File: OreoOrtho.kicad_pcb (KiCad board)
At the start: 2 copper layers, 57.1 x 39.3 mm, 36 parts, among them SW1 MXSwitch, SW2 MXSwitch, SW3 MXSwitch, SW4 MXSwitch, SW5 MXSwitch, SW6 MXSwitch, U1 ATmega32U2-AU, U2 PRTR5V0U2X, Y1 16MHz

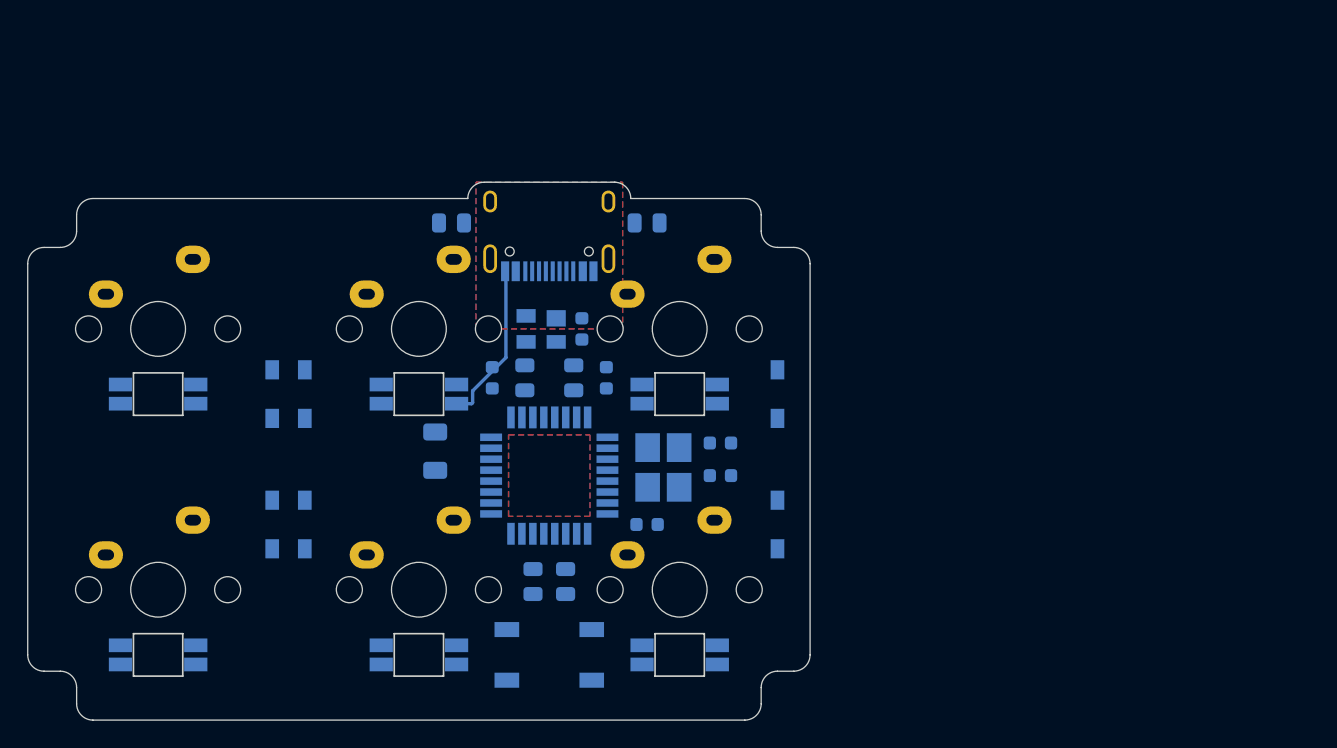
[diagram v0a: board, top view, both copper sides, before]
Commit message: made gerbers
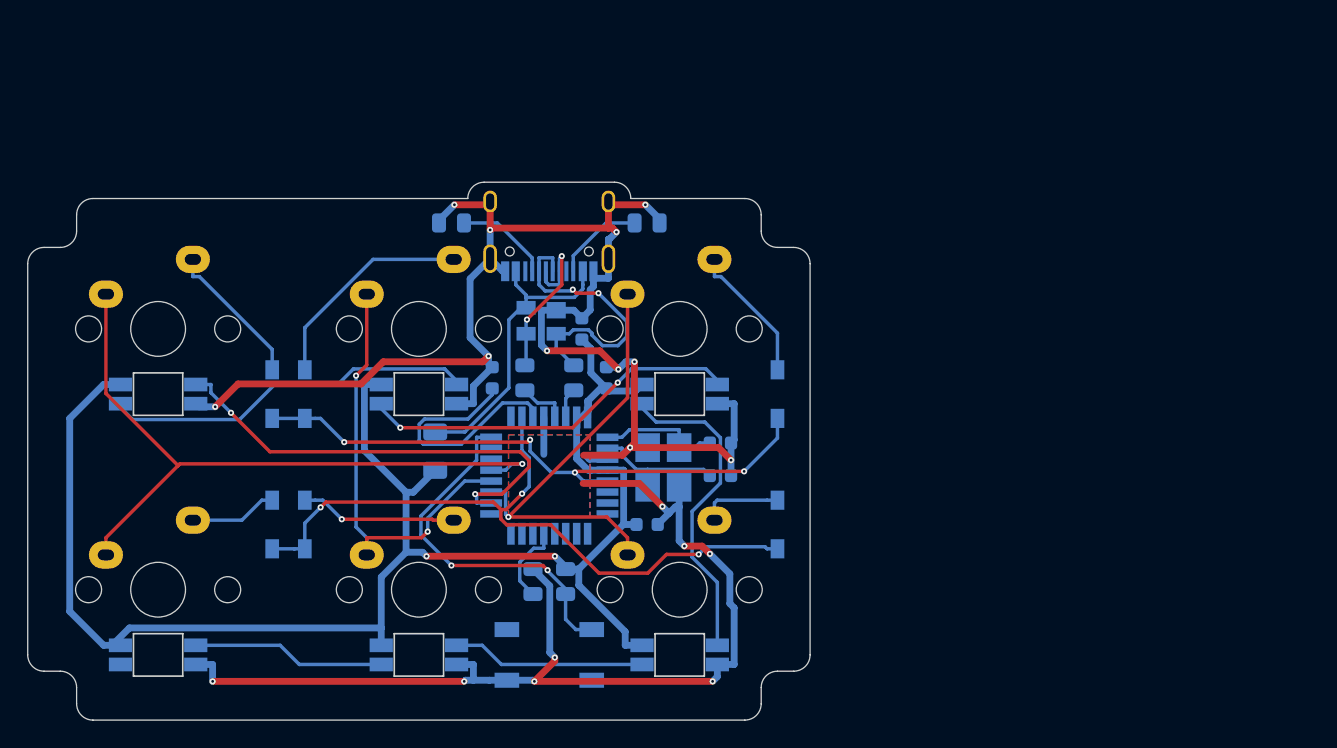
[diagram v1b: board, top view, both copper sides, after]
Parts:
- USB1: value HRO-TYPE-C-31-M-12 -> HRO-TYPE-C-31-M-12-Assembly
- moved U2 0.60 mm to (142.3, 56.6)
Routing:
- net GND: track 11.8 -> 193.8 mm, vias 0 -> 19
- net +5V: track 0.00 -> 118.4 mm, vias 0 -> 2
- net Col0: track 0.00 -> 51.1 mm, vias 0 -> 1
- net Row1: track 0.00 -> 50.9 mm, vias 0 -> 3
- net Row0: track 0.00 -> 44.3 mm, vias 0 -> 4
- net LED: track 0.00 -> 34.0 mm, vias 0 -> 2
- net Col2: track 0.00 -> 33.4 mm, vias 0 -> 1
- net Col1: track 0.00 -> 32.3 mm, vias 0 -> 2
- net Net-(LED2-Pad2): track 0.00 -> 27.9 mm, vias 0 -> 2
- net Net-(LED1-Pad2): track 0.00 -> 27.3 mm
- net Net-(R1-Pad1): track 0.00 -> 26.5 mm, vias 0 -> 2
- net Net-(LED3-Pad2): track 0.00 -> 23.7 mm
- net VCC: track 0.00 -> 22.1 mm
- net Net-(R5-Pad2): track 0.00 -> 21.6 mm, vias 0 -> 2
- net Net-(C3-Pad2): track 0.00 -> 18.3 mm
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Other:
- net class Default: clearance 0.2 -> 0.13; trace_width 0.25 -> 0.254; via_dia 0.8 -> 0.45; via_drill 0.4 -> 0.2
- net class thick added: clearance 0.13, trace_width 0.5, via_dia 0.45, via_drill 0.2
- rule trace_clearance: 0.2 -> 0.13
- rule trace_min: 0.2 -> 0.13
- rule via_min_drill: 0.3 -> 0.2
- rule via_min_size: 0.4 -> 0.45

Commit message: route ver1
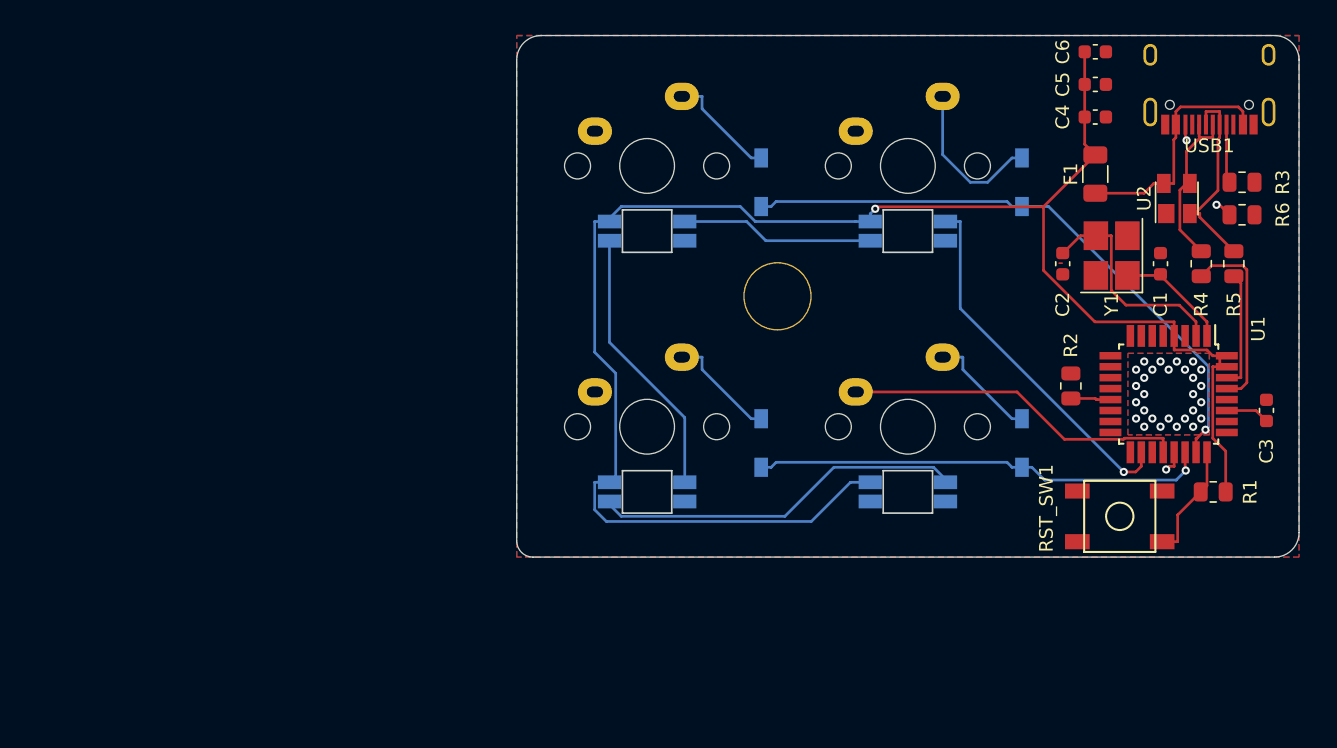
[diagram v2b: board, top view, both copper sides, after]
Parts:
- removed D5, D6: D, kbd:D3_SMD_v2
- removed LED5, LED6: YS-SK6812MINI-E, kbd:YS-SK6812MINI-E
- removed SW5, SW6: MXSwitch, kbd:CherryMX_1u
- added H1: MountingHole, kbd:HOLE, F.Cu at (159.5, 54.8)
- C1, C2, C3, C4, C5, C6, F1, R1, R2, R3, R4, R5, R6, RST_SW1, U1, U2, Y1: moved to F.Cu
- USB1: value HRO-TYPE-C-31-M-12-Assembly -> HRO-TYPE-C-31-M-12; moved to F.Cu
- moved R3 57.8 mm to (193.5, 46.4), turned to 0 degrees
- moved C3 56.6 mm to (195.3, 63.1)
- moved LED1 56.0 mm to (169.1, 50.0)
- moved SW4 56.0 mm to (169.1, 64.3)
- moved D4 55.1 mm to (177.4, 65.5)
- moved D2 54.6 mm to (177.4, 46.4)
- moved F1 52.3 mm to (182.8, 45.8), turned to 270 degrees
- moved R4 50.1 mm to (190.5, 52.4)
- moved USB1 49.4 mm to (191.1, 34.5), turned to 180 degrees
- moved R5 48.9 mm to (192.9, 52.4)
- moved R1 47.8 mm to (191.4, 69.1), turned to 0 degrees
- moved C6 47.6 mm to (182.8, 36.9)
- moved U2 47.3 mm to (188.7, 47.6), turned to 90 degrees
- moved U1 45.6 mm to (188.1, 61.9), turned to 270 degrees
- moved R6 43.5 mm to (193.5, 48.8)
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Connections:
- D3 pad 1: Row0 -> Row1
- LED4 pad 2: Net-(LED4-Pad2) -> (no net)
- SW3 pad 1: Col2 -> Col0
- SW4 pad 1: Col0 -> Col1
- U1 pad 19: Col2 -> (no net)
- U1 pad 22: (no net) -> Row1
- U1 pad 23: (no net) -> Row0
- U1 pad 26: Row1 -> (no net)
- U1 pad 5: Row0 -> (no net)
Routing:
- net GND: track 193.8 -> 0.22 mm, vias 19 -> 28
- net Col2: track 33.4 -> 0.00 mm, vias 1 -> 0
- net Net-(R1-Pad1): track 26.5 -> 8.55 mm, vias 2 -> 0
- net Row1: track 50.9 -> 33.3 mm, vias 3 -> 1
- net Net-(C3-Pad2): track 18.3 -> 3.21 mm
- net Net-(LED4-Pad2): track 14.1 -> 0.00 mm
- net Net-(LED5-Pad2): track 14.1 -> 0.00 mm
- net Col0: track 51.1 -> 64.8 mm
- net Net-(LED1-Pad2): track 27.3 -> 14.1 mm
- net Col1: track 32.3 -> 44.0 mm, vias 2 -> 0
- net Net-(D5-Pad2): track 11.5 -> 0.00 mm, vias 1 -> 0
- net D+: track 3.63 -> 13.7 mm
- net Net-(LED2-Pad2): track 27.9 -> 19.9 mm, vias 2 -> 0
- net +5V: track 118.4 -> 125.6 mm, vias 2 -> 1
- net LED: track 34.0 -> 26.8 mm, vias 2 -> 1
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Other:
- board size 57.1 x 39.3 mm -> 57.2 x 38.1 mm
- copper layers 2 -> 4
- net class Default: clearance 0.13 -> 0.127; trace_width 0.254 -> 0.2; via_dia 0.45 -> 0.6; via_drill 0.2 -> 0.3
- net class thick: clearance 0.13 -> 0.127; trace_width 0.5 -> 0.4; via_dia 0.45 -> 0.6; via_drill 0.2 -> 0.3
- rule trace_clearance: 0.13 -> 0.127
- rule trace_min: 0.13 -> 0.127
- rule via_min_drill: 0.2 -> 0.3
- rule via_min_size: 0.45 -> 0.6

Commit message: reroute
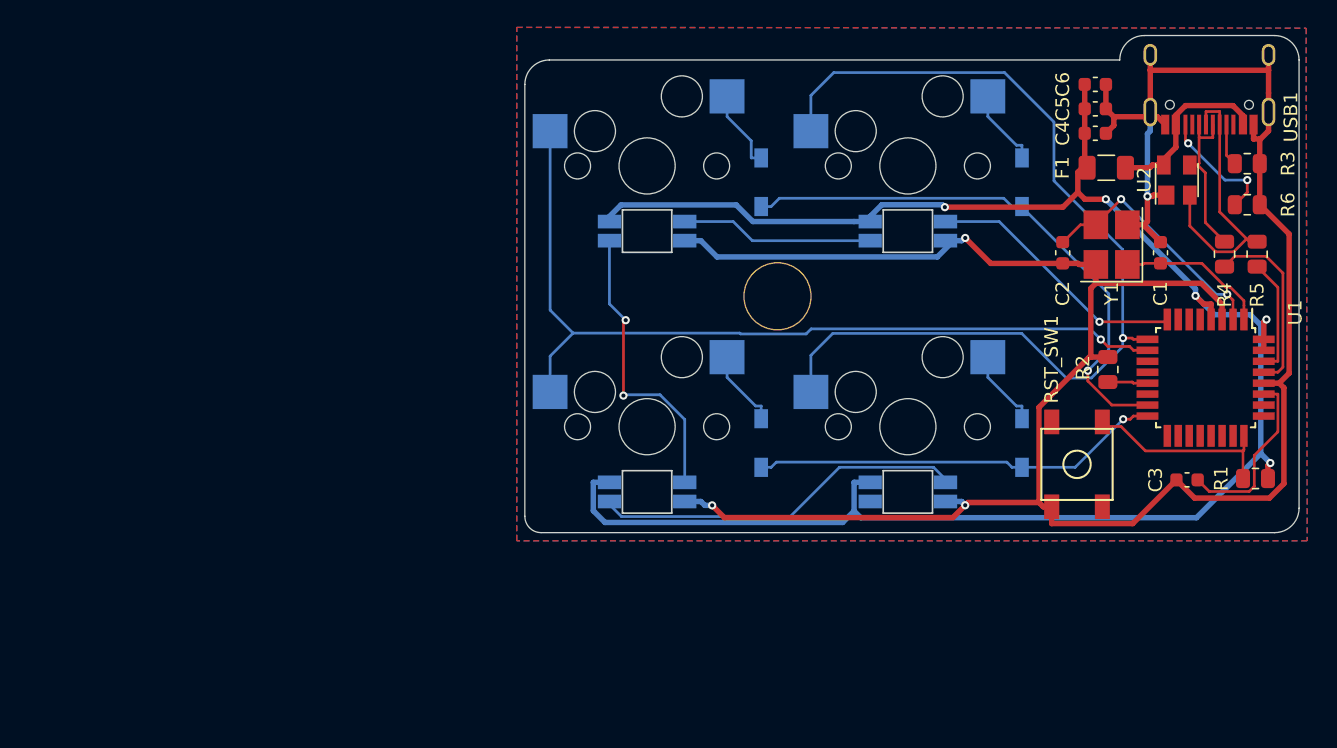
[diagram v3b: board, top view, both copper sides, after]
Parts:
- SW1, SW2, SW3, SW4: footprint kbd:CherryMX_1u -> kbd:CherryMX_Hotswap
- moved C3 7.71 mm to (189.5, 68.2), turned to 0 degrees
- moved RST_SW1 4.92 mm to (181.4, 67.0), turned to 270 degrees
- moved R1 3.24 mm to (194.5, 68.1)
- moved R2 2.95 mm to (183.7, 60.1)
- moved U1 2.95 mm to (190.8, 60.7)
- moved C6 2.38 mm to (182.8, 39.3)
- moved R4 1.84 mm to (192.2, 51.7)
- moved R5 1.84 mm to (194.6, 51.7)
- moved C5 1.79 mm to (182.8, 41.1)
- moved R3 1.41 mm to (193.9, 45.1)
- moved U2 1.35 mm to (188.7, 46.3)
- moved C4 1.19 mm to (182.8, 42.9)
- moved F1 0.92 mm to (183.6, 45.4), turned to 0 degrees
- moved R6 0.83 mm to (193.9, 48.1)
- moved C1 0.80 mm to (187.5, 51.6)
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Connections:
- U1 pad 10: (no net) -> Col0
- U1 pad 12: (no net) -> Net-(U1-Pad12)
- U1 pad 15: (no net) -> Row0
- U1 pad 16: (no net) -> Row1
- U1 pad 18: LED -> (no net)
- U1 pad 20: Col1 -> (no net)
- U1 pad 21: Col0 -> (no net)
- U1 pad 22: Row1 -> (no net)
- U1 pad 23: Row0 -> (no net)
- U1 pad 8: (no net) -> LED
- U1 pad 9: (no net) -> Col1
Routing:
- net GND: track 0.22 -> 183.4 mm, vias 28 -> 4
- net Col1: track 44.0 -> 71.3 mm, vias 0 -> 1
- net +5V: track 125.6 -> 137.9 mm, vias 1 -> 5
- net Net-(C3-Pad2): track 3.21 -> 13.1 mm
- net LED: track 26.8 -> 19.3 mm
- net Net-(D2-Pad2): track 11.6 -> 5.76 mm
- net Net-(R5-Pad2): track 14.7 -> 20.5 mm
- net Net-(R1-Pad1): track 8.55 -> 14.3 mm
- net VCC: track 17.5 -> 13.2 mm
- net Row0: track 44.5 -> 40.7 mm
- net Row1: track 33.3 -> 30.1 mm
- net Net-(C1-Pad2): track 8.33 -> 11.0 mm
- net Net-(D3-Pad2): track 8.19 -> 5.76 mm
- net Net-(D4-Pad2): track 8.19 -> 5.76 mm
- net Net-(C2-Pad2): track 16.2 -> 18.5 mm, vias 0 -> 2
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- added copper zone on B.Cu, net (none)
- added copper zone on F.Cu, net (none)
- removed copper zone on B.Cu, net GND
- removed copper zone on F.Cu, net GND
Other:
- board size 57.2 x 38.1 mm -> 56.6 x 36.3 mm
- copper layers 4 -> 2
